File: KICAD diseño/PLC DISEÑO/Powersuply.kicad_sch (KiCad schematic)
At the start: 5 parts, among them U2 AP63203WU

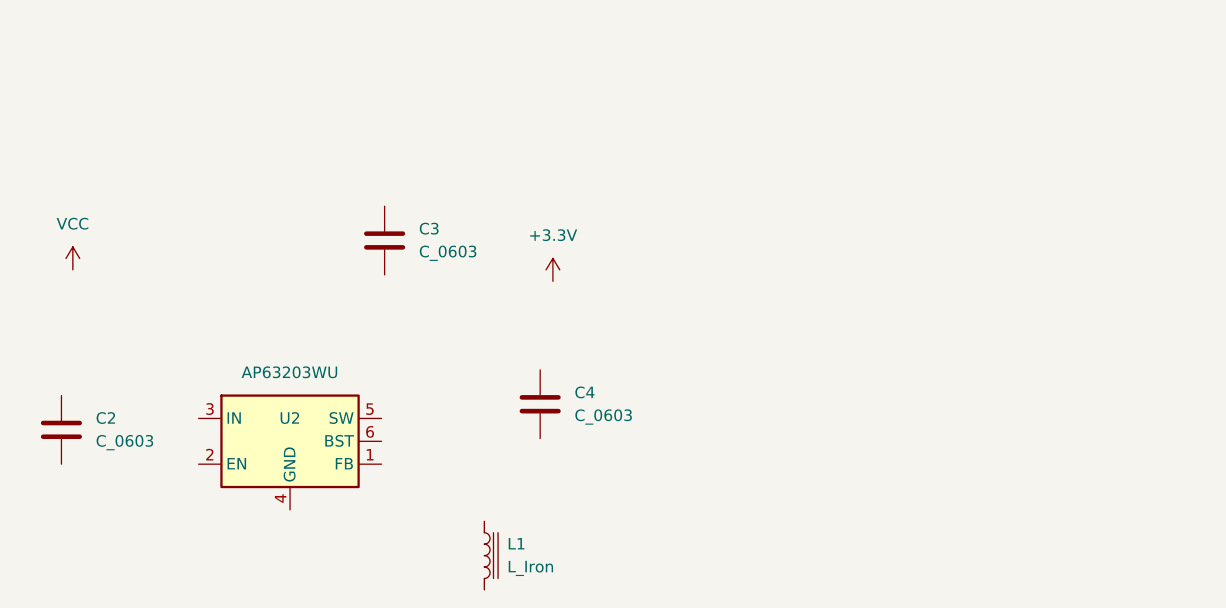
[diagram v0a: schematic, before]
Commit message: Update
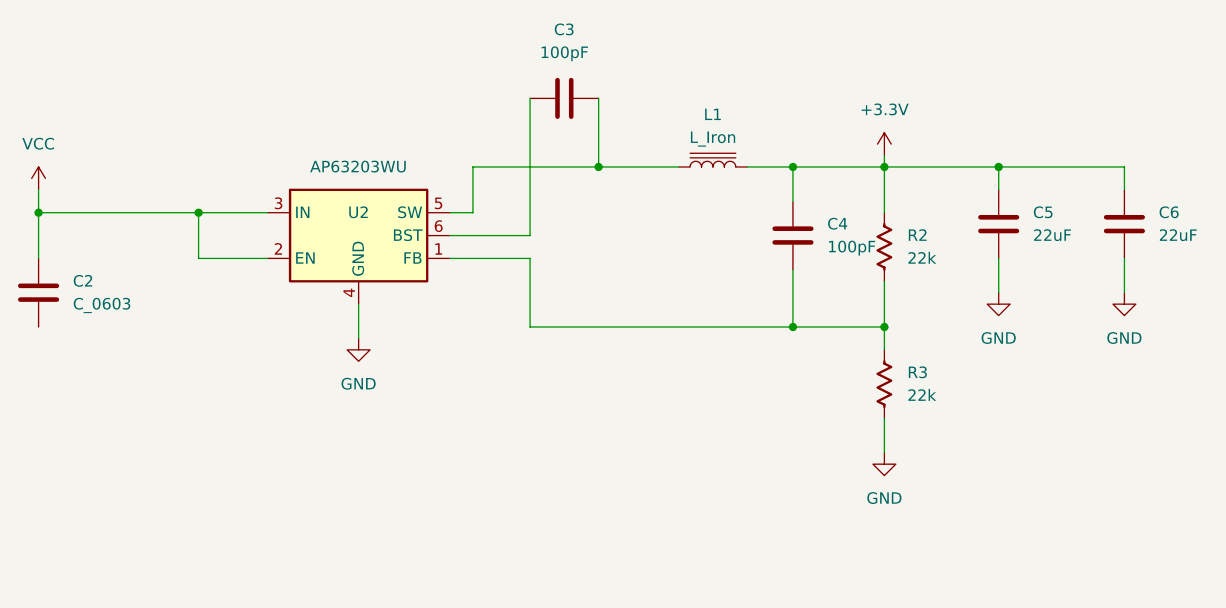
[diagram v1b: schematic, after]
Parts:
- added C5, C6: 22uF, PCM_Capacitor_SMD_AKL:C_0603_1608Metric, symbol PCM_Capacitor_AKL:C_0603
- added R2, R3: 22k, PCM_Resistor_SMD_AKL:R_0603_1608Metric, symbol PCM_Resistor_US_AKL:R_0603
- C3, C4: value C_0603 -> 100pF
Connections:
- net +3.3V: now also C4.1, L1.2, C5.1, C6.1, R2.1
- net VCC: now also C2.1, U2.2 (EN), U2.3 (IN)
- net at U2.1 (FB): now also C4.2, R2.2, R3.1
- net GND: now reaches U2.4 (GND)
- net GND: now also C5.2, C6.2, R3.2
- net at U2.5 (SW): now also C3.2, L1.1
- net at U2.6 (BST): now also C3.1
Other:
- moved on the sheet: C2, C3, C4, L1, U2
